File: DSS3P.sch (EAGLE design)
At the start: 289 parts, among them J1 J5MM

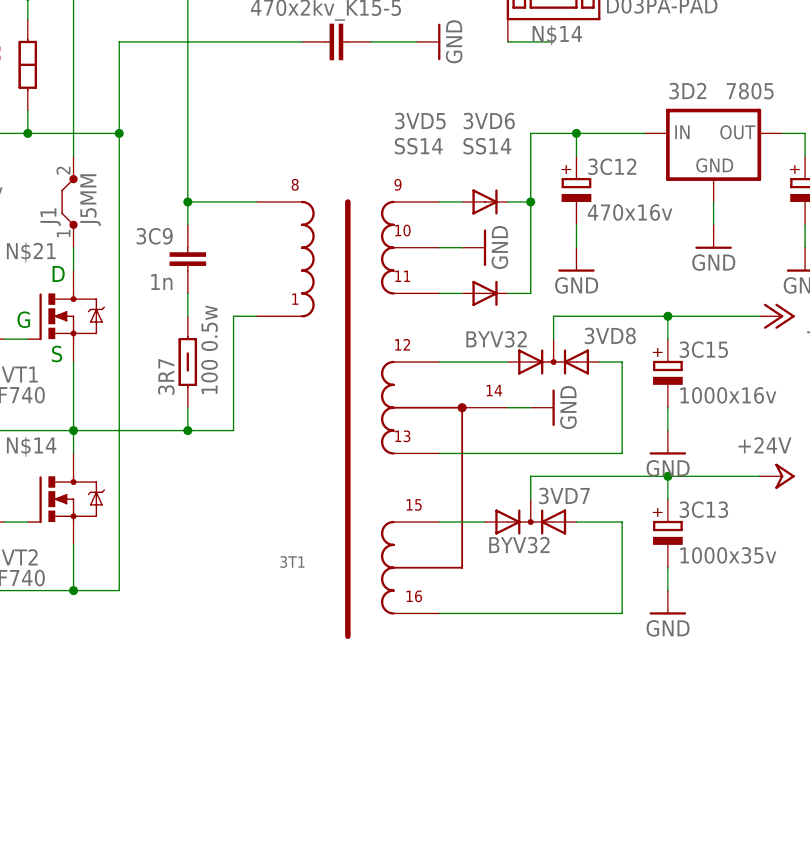
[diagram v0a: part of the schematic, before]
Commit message: .
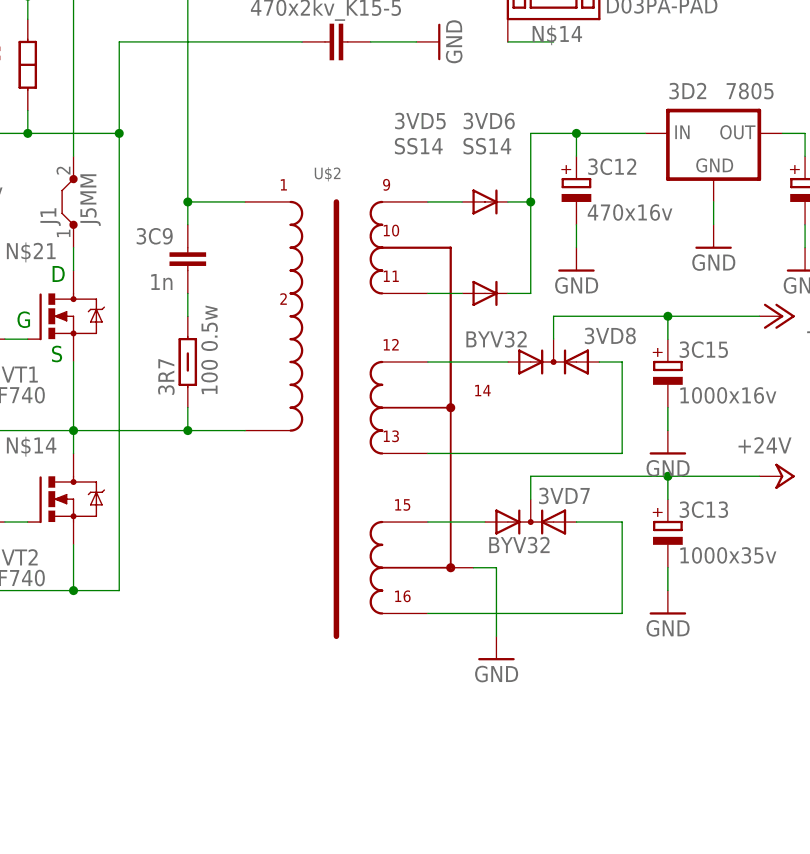
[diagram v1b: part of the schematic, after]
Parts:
- removed 3T1: TRANS_ER35/20/11, DSS:TRANS_ER35/20/11
- added U$2: TRANS_ER38, DSS0:TRANS_ER38
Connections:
- net GND: now also U$2.GND; no longer 3T1.P$4, 3T1.P$8
- net N$100: now also U$2.5-2; no longer 3T1.P$5
- net N$14: now also U$2.IN2; no longer 3T1.P$2
- net N$87: now also U$2.IN1; no longer 3T1.P$1
- net N$95: now also U$2.12-1; no longer 3T1.P$6
- net N$96: now also U$2.12-2; no longer 3T1.P$7
- net N$97: now also U$2.24-1; no longer 3T1.P$9
- net N$98: now also U$2.24-2; no longer 3T1.P$10
- net N$99: now also U$2.5-1; no longer 3T1.P$3
